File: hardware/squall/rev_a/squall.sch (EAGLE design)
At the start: 38 parts, among them J1 HIROSE-DF40C-10DP-0.4V, J2 HIROSE-DF40C-10DP-0.4V, J3 MICRO_USB_B_JST_MC5BR3-M404-4S, J4 TC2030-JLINK-NL, U1 NRF51822QF, U2 FT232RQ, X1 16MHz, X2 ABS05-32.768KHZ-9-T

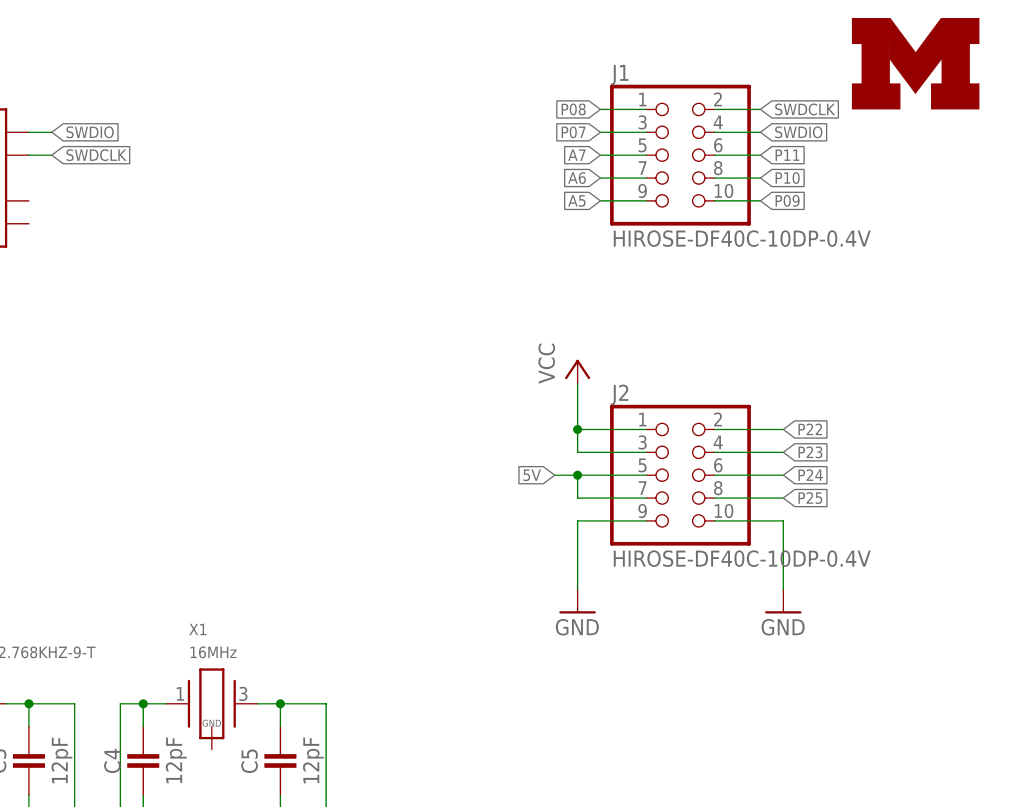
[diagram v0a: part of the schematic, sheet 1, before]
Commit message: squall rev a ready to ship
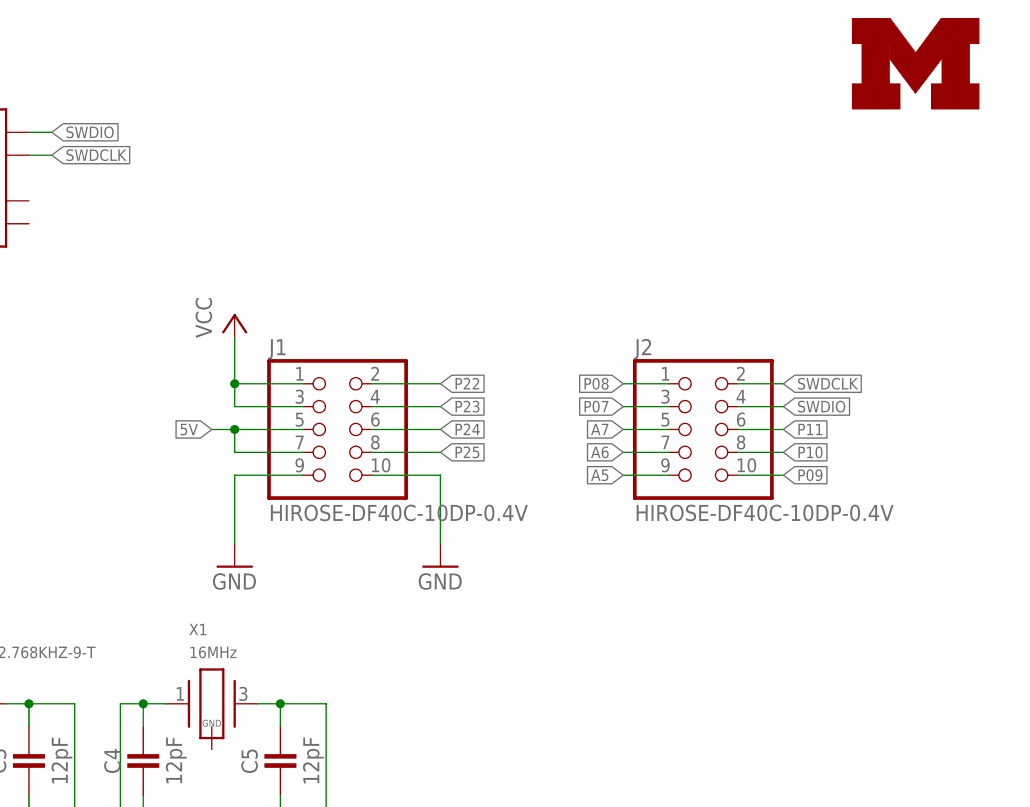
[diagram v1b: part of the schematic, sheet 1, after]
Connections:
- net 5V: now also J1.5, J1.7; no longer J2.5, J2.7
- net A5: now also J2.9; no longer J1.9
- net A6: now also J2.7; no longer J1.7
- net A7: now also J2.5; no longer J1.5
- net GND: now also J1.10, J1.9; no longer J2.10, J2.9
- net P07: now also J2.3; no longer J1.3
- net P08: now also J2.1; no longer J1.1
- net P09: now also J2.10; no longer J1.10
- net P10: now also J2.8; no longer J1.8
- net P11: now also J2.6; no longer J1.6
- net P22: now also J1.2; no longer J2.2
- net P23: now also J1.4; no longer J2.4
- net P24: now also J1.6; no longer J2.6
- net P25: now also J1.8; no longer J2.8
- net SWDCLK: now also J2.2; no longer J1.2
- net SWDIO: now also J2.4; no longer J1.4
- net VCC: now also J1.1, J1.3; no longer J2.1, J2.3
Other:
- note added: "Batteries"
- note added: "FTDI Circuit for UART Programming and Communication"
- note added: "JTAG Connection"
- note added: "Left Header"
- note added: "Note: Only one battery can be connected at a time. If BAT1 is connected, do not populate D2 or R2. If BAT2 is connected, D2 and R2 must be populated for recharging."
- note added: "Reset Switch"
- note added: "Right Header"
- moved on the sheet: J1, J2
